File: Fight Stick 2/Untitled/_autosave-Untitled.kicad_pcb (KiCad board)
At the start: 2 copper layers, 146.2 x 62.1 mm, 18 parts, among them U1 Elite-C

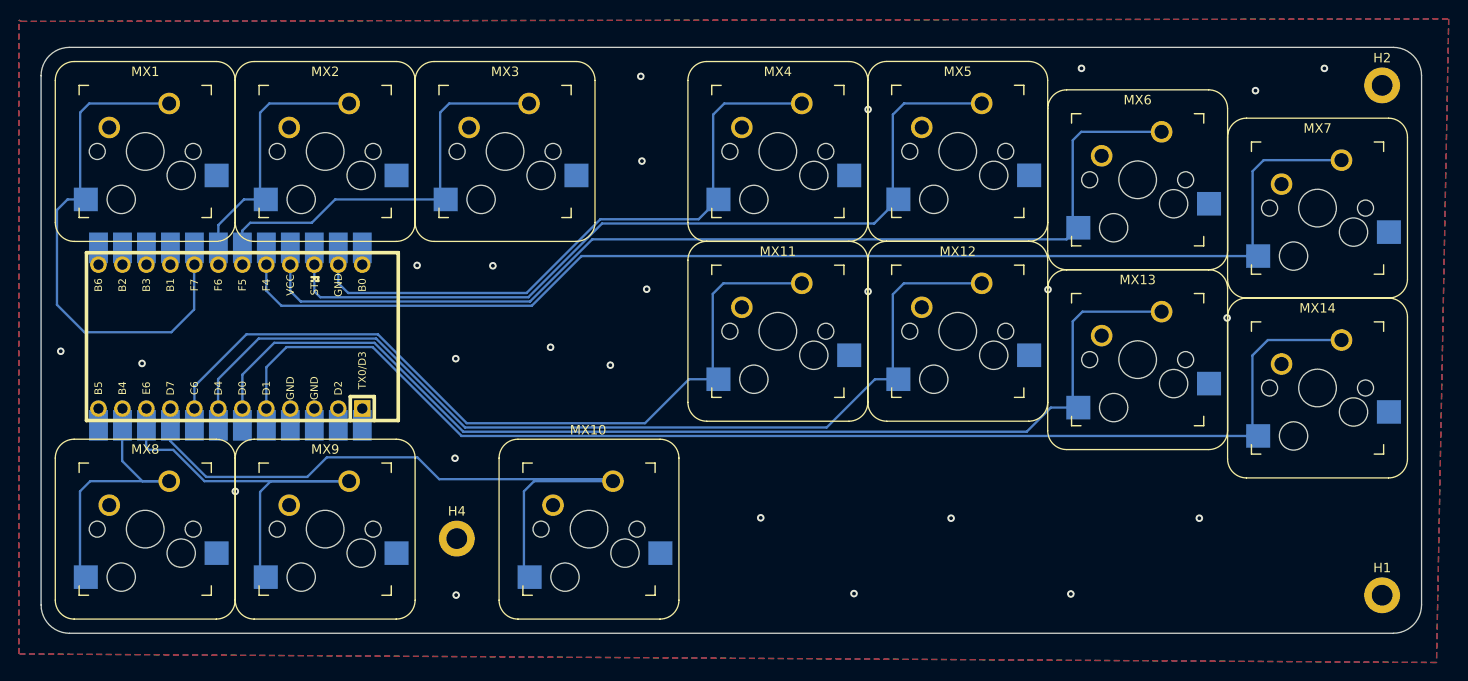
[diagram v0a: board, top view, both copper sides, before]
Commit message: second version upload
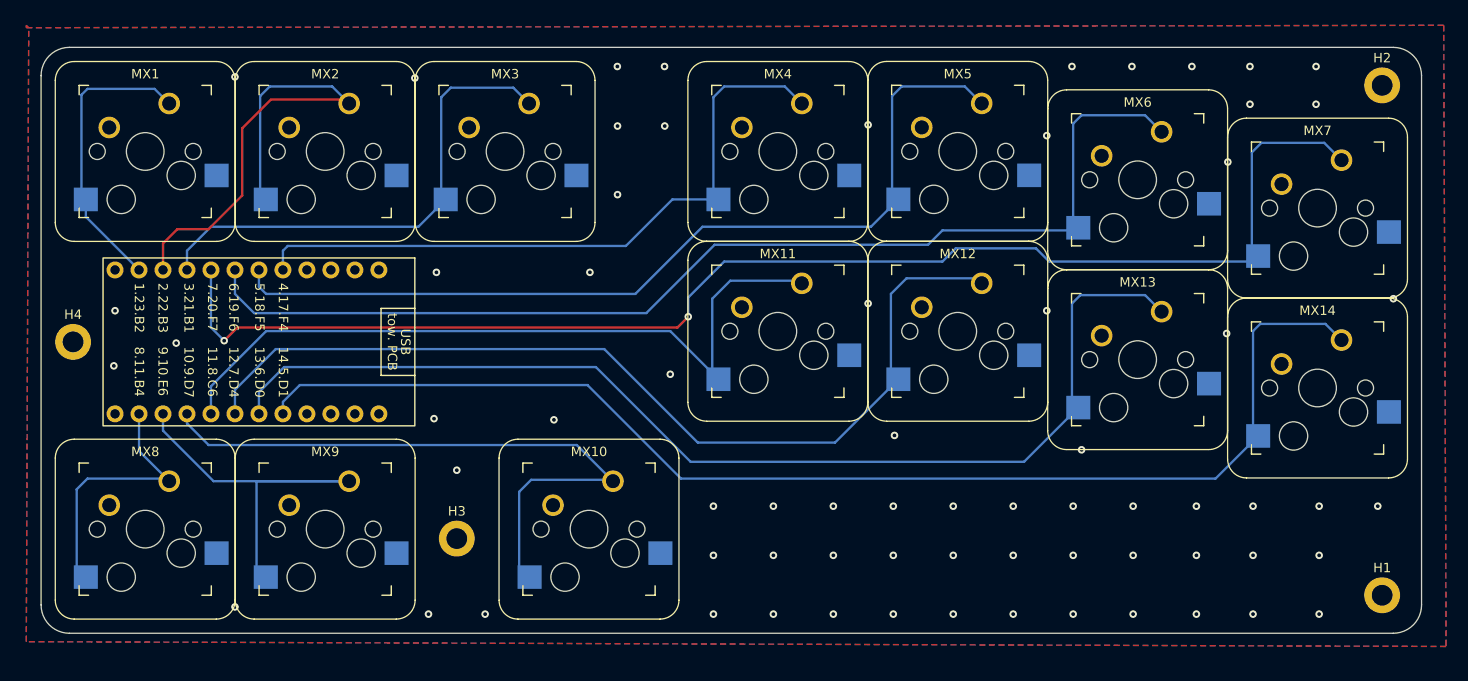
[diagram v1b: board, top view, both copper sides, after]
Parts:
- removed U1: Elite-C, Keebio-Parts.pretty-master:Elite-C-castellated-24pin-holes
- added H4: MountingHole, MountingHole:MountingHole_2.2mm_M2_DIN965_Pad, F.Cu at (78.4, 74.2)
- added U2: ProMicro, PCM_marbastlib-xp-promicroish:ProMicro_Reversible_Single, B.Cu at (96.8, 74.2)
- MX1, MX10, MX11, MX12, MX13, MX14, MX2, MX3, MX4, MX5, MX6, MX7, MX8, MX9: footprint keyswitches.pretty-2.1:Kailh_socket_MX_optional -> Fight Stick 2:MX_optional
- renumbered H4 to H3
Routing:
- net MX2: track 30.0 -> 54.9 mm
- net MX1: track 54.3 -> 31.3 mm
- net MX7: track 129.8 -> 145.6 mm, vias 0 -> 2
- net MX6: track 109.2 -> 118.2 mm
- net MX5: track 88.4 -> 95.8 mm
- net MX3: track 46.2 -> 53.1 mm
- net MX4: track 65.8 -> 72.0 mm
- net MX11: track 85.6 -> 80.4 mm
- net MX10: track 73.0 -> 68.7 mm
- net MX9: track 46.3 -> 44.1 mm
- net MX8: track 30.7 -> 28.5 mm
- net MX12: track 102.1 -> 101.4 mm
- net MX14: track 133.5 -> 133.0 mm
- net GND: vias 25 -> 69
